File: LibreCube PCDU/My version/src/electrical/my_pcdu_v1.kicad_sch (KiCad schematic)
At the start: 117 parts, among them J1 Conn_01x02, J2 Conn_01x02, J3 Conn_01x02, J4 Conn_01x02, J5 Conn_01x02, J6 Conn_01x02, J7 Conn_01x02, J8 USB_C_Receptacle_PowerOnly_6P, M1 MountingHole, M2 MountingHole, M3 MountingHole, M4 MountingHole, U1 TPS2034, U10 TPS2034, U11 TPS61032, U12 TPS61032, U13 TPS2034, U14 TPS2034, U15 TPS2034, U16 TPS2034, U2 TPS2034, U3 TPS2034, U4 TPS2034, U5 TPS61032, U6 TPS61032, U7 bq24002, U8 bq24002, U9 TPS2034

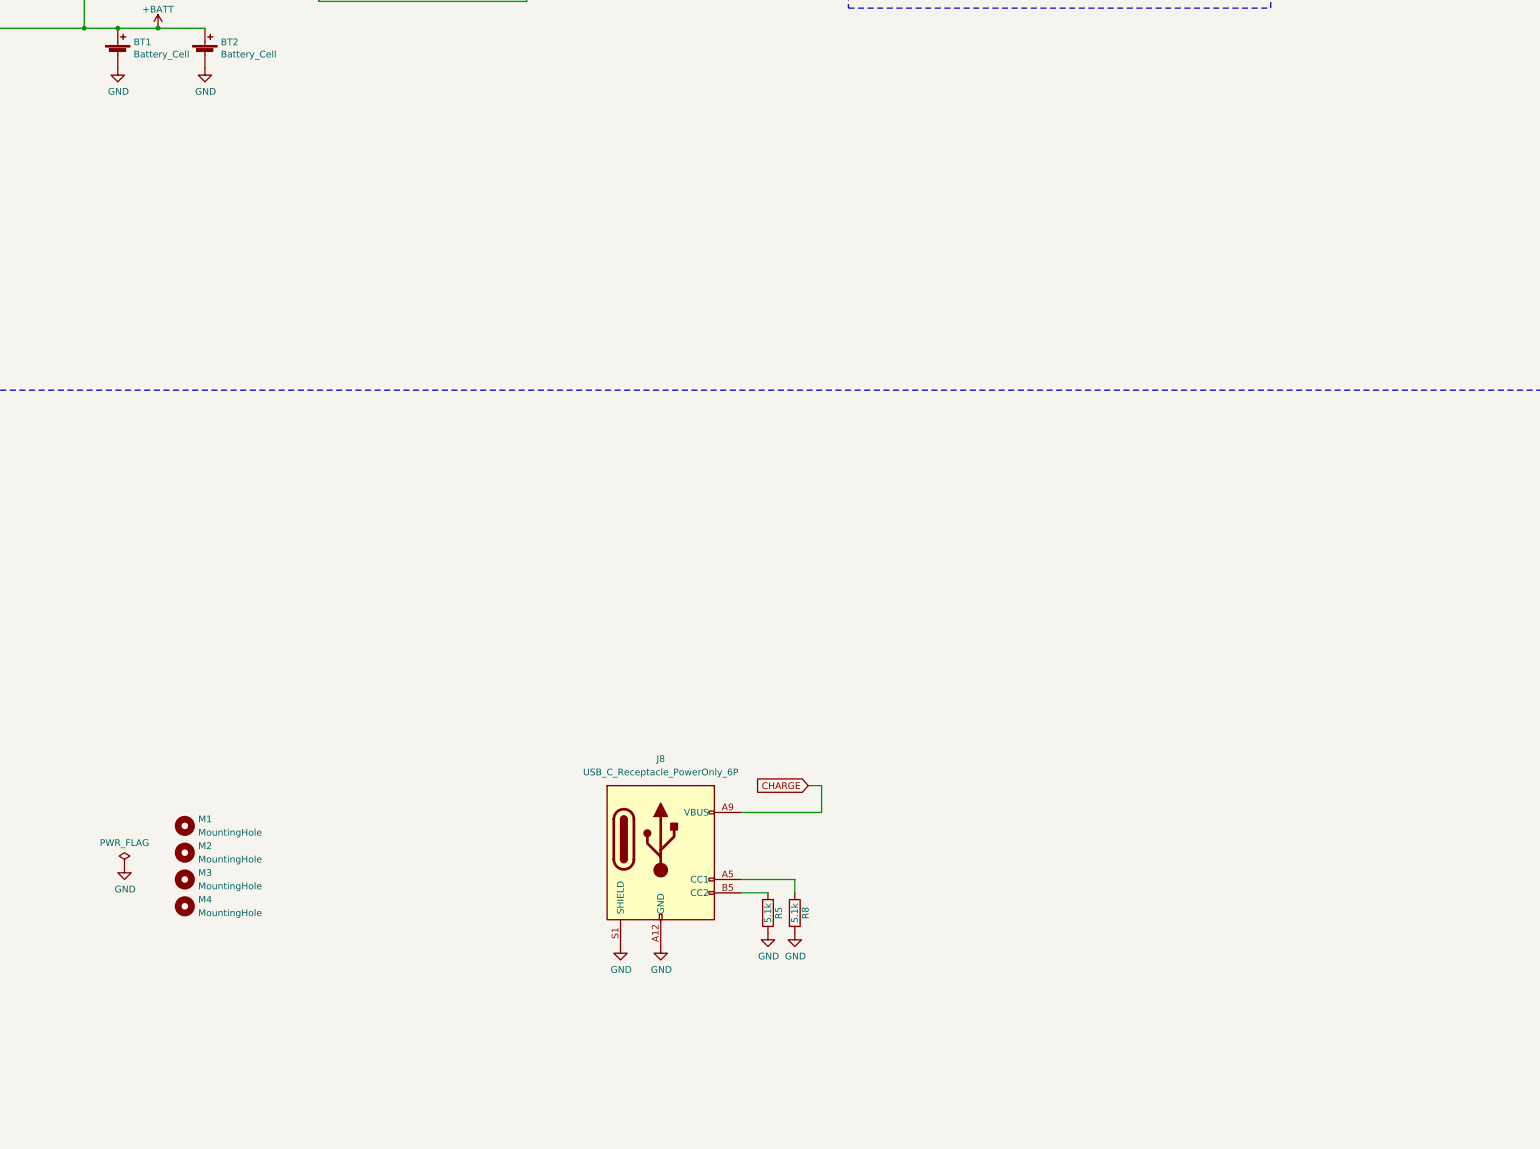
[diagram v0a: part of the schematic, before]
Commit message: New components
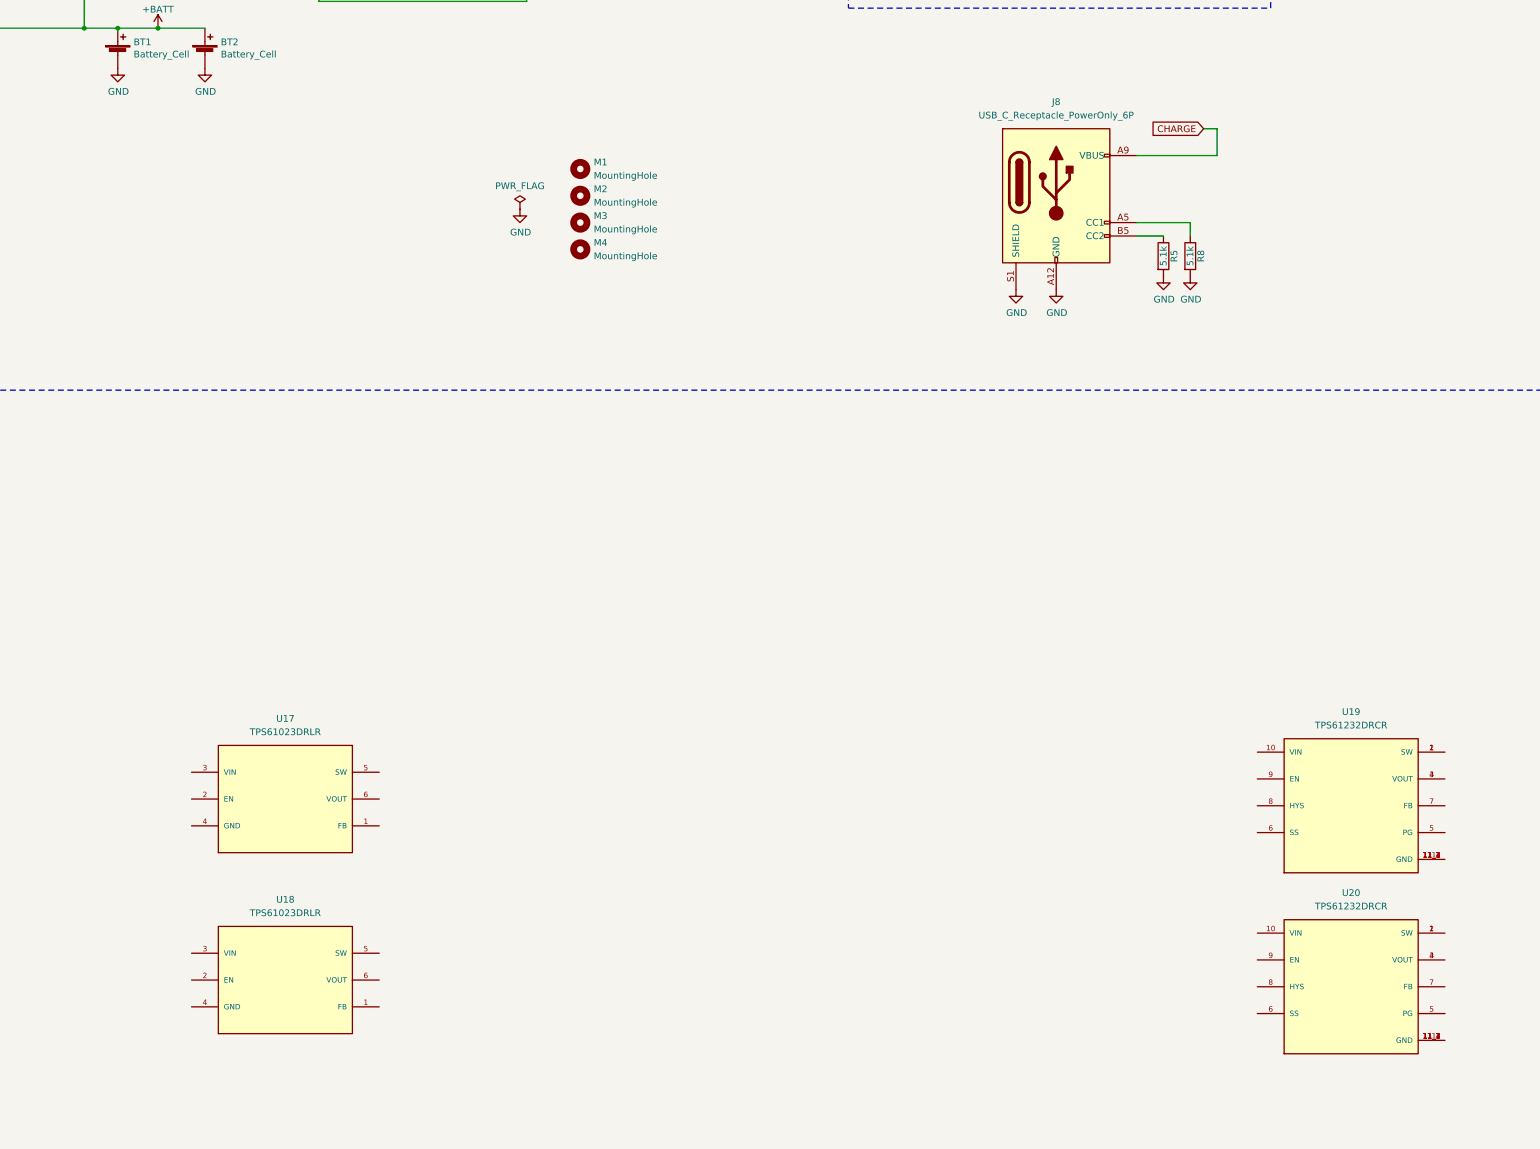
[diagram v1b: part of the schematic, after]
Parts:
- added U17, U18: TPS61023DRLR, TPS61023DRLR:DRL0006A, symbol TPS61023DRLR:TPS61023DRLR
- added U19, U20: TPS61232DRCR, TPS61232DRCR:VREG_TPS61232DRCR, symbol TPS61232DRCR:TPS61232DRCR
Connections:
- new net: U20.1 (SW), U20.2 (SW)
- new net: U20.11 (GND), U20.11_1 (GND), U20.11_2 (GND), U20.11_3 (GND), U20.11_4 (GND)
- new net: U20.3 (VOUT), U20.4 (VOUT)
- new net: U19.1 (SW), U19.2 (SW)
- new net: U19.11 (GND), U19.11_1 (GND), U19.11_2 (GND), U19.11_3 (GND), U19.11_4 (GND)
- new net: U19.3 (VOUT), U19.4 (VOUT)
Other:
- moved on the sheet: J8, M1, M2, M3, M4, R5, R8
